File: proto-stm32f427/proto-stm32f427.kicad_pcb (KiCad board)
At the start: 2 copper layers, 54.6 x 66.7 mm, 37 parts, among them J1 Left, J2 Micro_SD_Card, J3 USB, J4 Debug, J5 Right, U1 NCV5501, U2 STM32F427VGTx, Y1 8 MHz

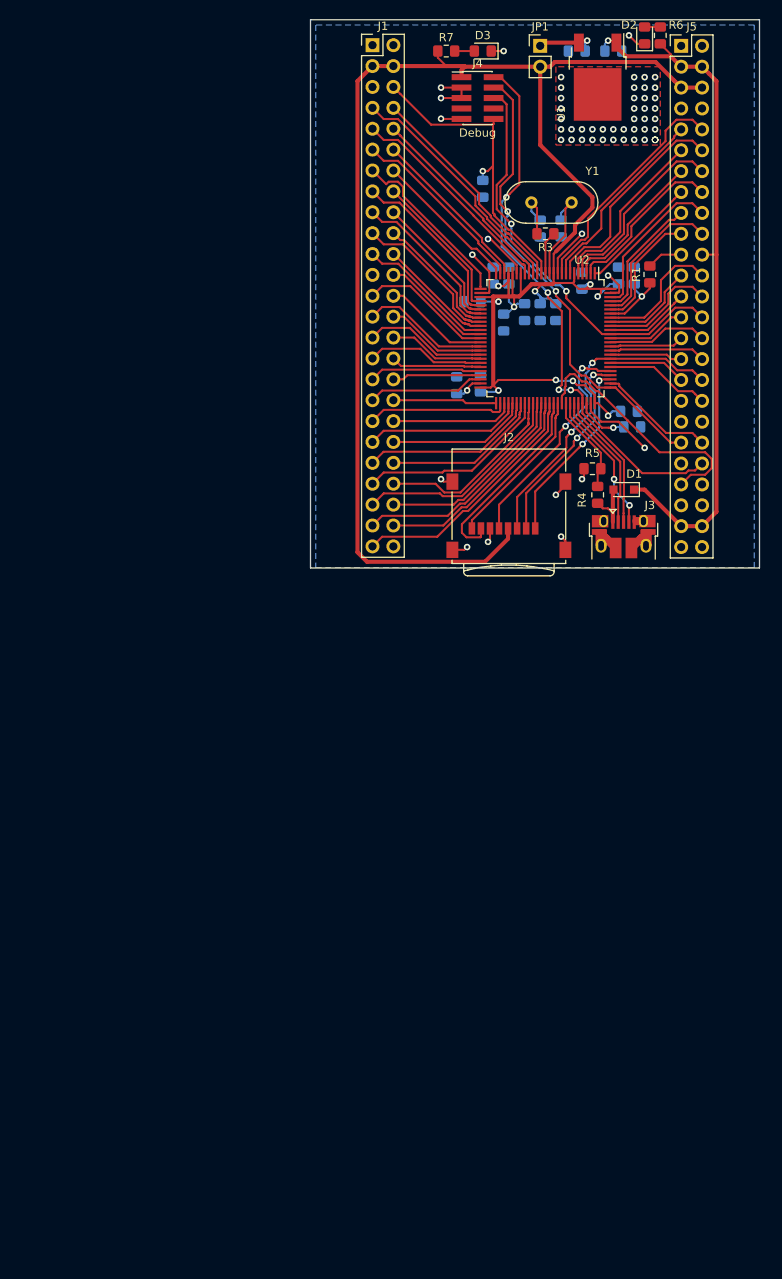
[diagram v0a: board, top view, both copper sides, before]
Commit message: WIP updates for proto board to make smaller
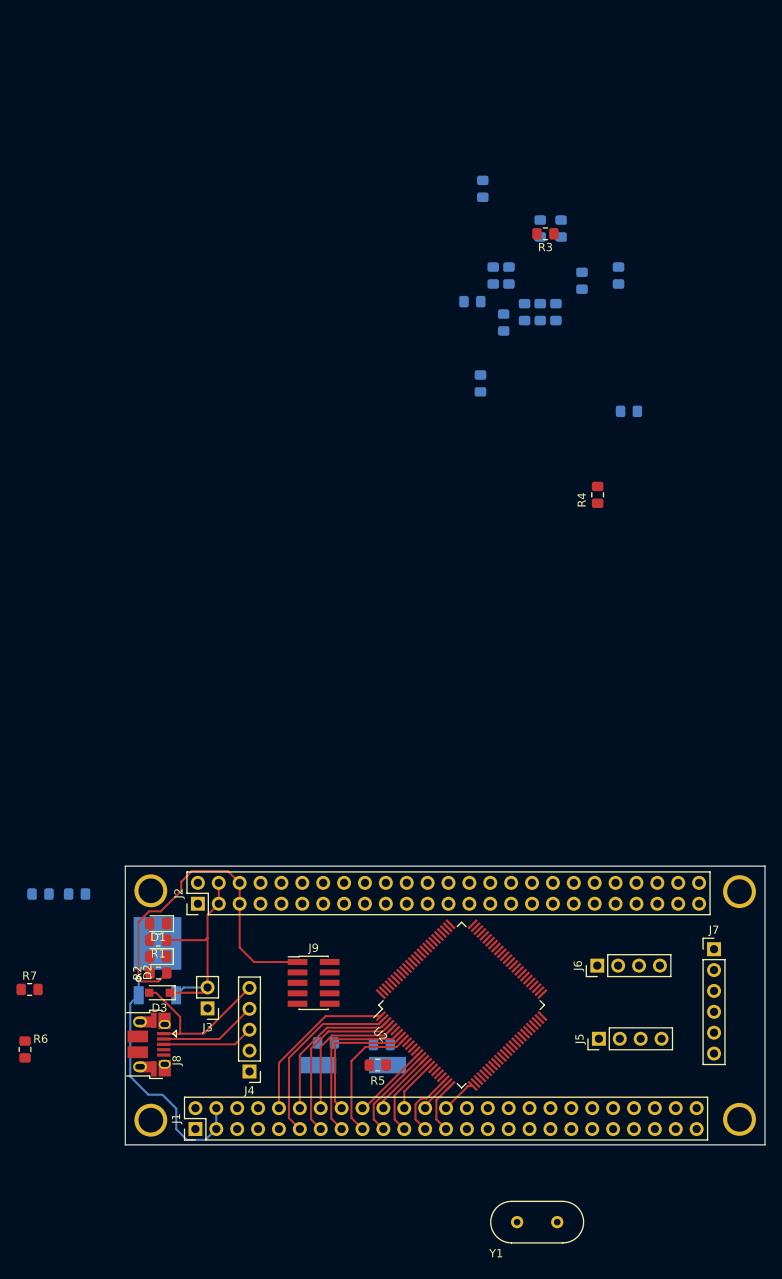
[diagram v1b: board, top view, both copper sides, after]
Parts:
- removed JP1: Idd, Connector_PinHeader_2.54mm:PinHeader_1x02_P2.54mm_Vertical
- added J6: IGNITION, Connector_PinHeader_2.54mm:PinHeader_1x04_P2.54mm_Vertical, F.Cu at (93.3, 136.0)
- added J7: SPI, Connector_PinHeader_2.54mm:PinHeader_1x06_P2.54mm_Vertical, F.Cu at (107.5, 134.0)
- added J8: USB, Connector_USB:USB_Micro-B_Amphenol_10103594-0001LF_Horizontal, F.Cu at (38.8, 145.6)
- added J9: Debug, Connector_PinHeader_1.27mm:PinHeader_2x05_P1.27mm_Vertical_SMD, F.Cu at (58.8, 138.1)
- added REF**: MountingHole_2.5mm_Pad, MountingHole:MountingHole_2.5mm_Pad, F.Cu at (110.6, 127.0)
- added REF**: MountingHole_2.5mm_Pad, MountingHole:MountingHole_2.5mm_Pad, F.Cu at (39.0, 154.8)
- added REF**: MountingHole_2.5mm_Pad, MountingHole:MountingHole_2.5mm_Pad, F.Cu at (110.6, 154.7)
- added REF**: MountingHole_2.5mm_Pad, MountingHole:MountingHole_2.5mm_Pad, F.Cu at (39.0, 126.9)
- added REF**: Crystal_SMD_HC49-SD, Crystal:Crystal_SMD_HC49-SD, B.Cu at (63.5, 148.1)
- C3, C5: value 16 pF -> 2.2 uF
- C4, C6: value 2.2 uF -> 16 pF
- D1: value BAT48JFILM -> LED; footprint Diode_SMD:D_SOD-323_HandSoldering -> LED_SMD:LED_0805_2012Metric_Pad1.15x1.40mm_HandSolder
- D3: value LED -> BAT48JFILM; footprint LED_SMD:LED_0805_2012Metric_Pad1.15x1.40mm_HandSolder -> Diode_SMD:D_SOD-323_HandSoldering
- J2: value Micro_SD_Card -> Right; footprint Connector_Card:microSD_HC_Wuerth_693072010801 -> Connector_PinHeader_2.54mm:PinHeader_2x25_P2.54mm_Vertical
- J3: value USB -> POWER; footprint Connector_USB:USB_Micro-B_Amphenol_10103594-0001LF_Horizontal -> Connector_PinHeader_2.54mm:PinHeader_1x02_P2.54mm_Vertical
- J4: value Debug -> EXTUSB; footprint Connector_PinHeader_1.27mm:PinHeader_2x05_P1.27mm_Vertical_SMD -> Connector_PinHeader_2.54mm:PinHeader_1x05_P2.54mm_Vertical
- J5: value Right -> FUEL; footprint Connector_PinHeader_2.54mm:PinHeader_2x25_P2.54mm_Vertical -> Connector_PinHeader_2.54mm:PinHeader_1x04_P2.54mm_Vertical
- R1: value 1k -> 220
- R2: value 100k -> 220; moved to F.Cu
- R3: value 220 -> 1k
- R4: value 4.7k -> 100k
- R5: value 10k -> 220
- R6: value 220 -> 4.7k
- R7: value 220 -> 10k
- U1: moved to B.Cu
- moved R6 145.5 mm to (23.7, 146.2)
- moved J1 133.6 mm to (44.4, 155.9), turned to 90 degrees
- moved D2 126.7 mm to (39.9, 134.9), turned to 180 degrees
- moved R7 124.9 mm to (24.3, 138.9)
- moved Y1 124.2 mm to (83.5, 167.2), turned to 0 degrees
- moved J4 121.6 mm to (51.0, 148.9), turned to 180 degrees
- moved C1 121.5 mm to (30.0, 127.3)
- moved C2 121.5 mm to (25.6, 127.3)
- moved J5 121.2 mm to (93.5, 144.9), turned to 90 degrees
- moved D3 121.1 mm to (40.0, 139.3)
- moved U1 120.1 mm to (39.8, 135.4), turned to 90 degrees
- moved R2 102.7 mm to (39.9, 136.9), turned to 180 degrees
- moved R1 100.7 mm to (39.9, 132.9), turned to 180 degrees
- moved C6 83.7 mm to (60.3, 145.4)
- moved U2 81.7 mm to (76.8, 140.8), turned to 45 degrees
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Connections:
- C2 pad 1: /3v_regulated -> /3v_cpu
- C3 pad 1: GND -> Net-(C3-Pad1)
- C3 pad 2: /PH0 -> GND
- C4 pad 1: Net-(C4-Pad1) -> GND
- C4 pad 2: GND -> /PH0
- C5 pad 1: GND -> Net-(C5-Pad1)
- C5 pad 2: Net-(C5-Pad2) -> GND
- C6 pad 1: Net-(C6-Pad1) -> GND
- C6 pad 2: GND -> Net-(C6-Pad2)
- D1 pad 1: /5v -> GND
- D1 pad 2: /5v_usb -> Net-(D1-Pad2)
- D3 pad 1: GND -> /5v
- D3 pad 2: Net-(D3-Pad2) -> /5v_usb
- J1 pad 10: /PC2 -> /PE2
- J1 pad 11: /PA1 -> /PE3
- J1 pad 12: /PA0 -> /PE4
- J1 pad 13: /PA3 -> /PE5
- J1 pad 14: /PA2 -> /PE6
- J1 pad 15: /PA5 -> /PC13
- J1 pad 16: /PA4 -> /PC14
- J1 pad 17: /PA7 -> /PC15
- J1 pad 18: /PA6 -> /NRST
- J1 pad 19: /PC5 -> /PC0
- J1 pad 20: /PC4 -> /PC1
- J1 pad 21: /PB1 -> /PC2
- J1 pad 22: /PB0 -> /PC3
- J1 pad 23: GND -> /PA0
- J1 pad 24: /PB2 -> /PA1
- J1 pad 25: /PE7 -> /PA2
- J1 pad 26: /PE8 -> /PA3
- J1 pad 5: GND -> unconnected-(J1-Pad5)
- J1 pad 6: /NRST -> unconnected-(J1-Pad6)
- J1 pad 7: /PC1 -> unconnected-(J1-Pad7)
- J1 pad 8: /PC0 -> unconnected-(J1-Pad8)
- J1 pad 9: /PC3 -> unconnected-(J1-Pad9)
- J2 pad 1: /PC10 -> GND
- J2 pad 2: /PC11 -> GND
- J2 pad 3: /PD2 -> /5v
- J2 pad 4: /3v_cpu -> /5v
- J2 pad 5: /PC12 -> /3v_cpu
- J2 pad 6: GND -> /3v_cpu
- J2 pad 7: /PC8 -> unconnected-(J2-Pad7)
- J2 pad 8: /PC9 -> unconnected-(J2-Pad8)
- J2 pad 9: GND -> /PC14
- J3 pad 1: /5v_usb -> GND
- J3 pad 2: /PA11 -> /5v
- J4 pad 1: /3v_cpu -> GND
- J4 pad 2: /PA13 -> GND
- J4 pad 3: GND -> /PA12
- J4 pad 4: /PA14 -> /PA11
- J4 pad 5: GND -> /5v_usb
- J5 pad 1: GND -> /PD8
- J5 pad 2: GND -> /PD9
- J5 pad 3: /5v -> /PD10
- J5 pad 4: /5v -> /PD11
- R1 pad 1: Net-(R1-Pad1) -> /5v
- R1 pad 2: /BOOT0 -> Net-(D1-Pad2)
- R2 pad 1: GND -> /3v_cpu
- R2 pad 2: Net-(R1-Pad1) -> Net-(D2-Pad2)
- R3 pad 1: /PH1 -> Net-(R3-Pad1)
- R3 pad 2: Net-(C5-Pad2) -> /BOOT0
- R4 pad 1: /PA9 -> GND
- R4 pad 2: /5v_usb -> Net-(R3-Pad1)
- R5 pad 1: /PA9 -> /PH1
- R5 pad 2: GND -> Net-(C6-Pad2)
- R6 pad 1: /5v -> /PA9
- R6 pad 2: Net-(D2-Pad2) -> /5v_usb
- R7 pad 1: /3v_cpu -> /PA9
- R7 pad 2: Net-(D3-Pad2) -> GND
- U1 pad 3: /3v_regulated -> /3v_cpu
- U2 pad 49: Net-(C4-Pad1) -> Net-(C3-Pad1)
- U2 pad 73: Net-(C6-Pad1) -> Net-(C5-Pad1)
- U2 pad 94: Net-(R1-Pad1) -> Net-(R3-Pad1)
- Y1 pad 2: Net-(C5-Pad2) -> Net-(C6-Pad2)
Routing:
- net /3v_cpu: track 246.0 -> 73.2 mm, vias 10 -> 1
- net /PA13: track 67.4 -> 0.00 mm, vias 4 -> 0
- net GND: track 61.9 -> 0.00 mm, vias 58 -> 0
- net /5v: track 85.7 -> 27.5 mm, vias 1 -> 0
- net /PA14: track 57.0 -> 0.00 mm, vias 2 -> 0
- net /PB3: track 50.0 -> 0.00 mm, vias 2 -> 0
- net /PD2: track 39.1 -> 0.00 mm, vias 2 -> 0
- net /PA8: track 31.1 -> 0.00 mm
- net /PC7: track 30.6 -> 0.00 mm
- net /NRST: track 38.0 -> 9.55 mm, vias 1 -> 0
- net /PD15: track 28.4 -> 0.00 mm
- net /PC12: track 28.1 -> 0.00 mm, vias 2 -> 0
- net /PD13: track 26.5 -> 0.00 mm
- net /PC6: track 26.5 -> 0.00 mm
- net /PC11: track 24.6 -> 0.00 mm, vias 2 -> 0
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- removed copper zone on B.Cu, net GND
- removed copper zone on F.Cu, net GND
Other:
- board size 54.6 x 66.7 mm -> 77.8 x 33.9 mm
- net class Default removed
- board text removed: "3v"
- board text removed: "5v"
- board text removed: "A0"
- board text removed: "A1"
- board text removed: "A13"
- board text removed: "A14"
- board text removed: "A15"
- board text removed: "A2"
- board text removed: "A3"
- board text removed: "A4"
- board text removed: "A5"
- board text removed: "A6"
- board text removed: "A7"
- board text removed: "A8"
- board text removed: "B0"
- board text removed: "B1"
- board text removed: "B10"
- board text removed: "B11"
- board text removed: "B12"
- board text removed: "B13"
- board text removed: "B14"
- board text removed: "B15"
- board text removed: "B2"
- board text removed: "B3"
- board text removed: "B4"
- board text removed: "B5"
- board text removed: "B6"
- board text removed: "B7"
- board text removed: "B8"
- board text removed: "B9"
- board text removed: "BOOT0"
- board text removed: "C0"
- board text removed: "C1"
- board text removed: "C13"
- board text removed: "C14"
- board text removed: "C15"
- board text removed: "C2"
- board text removed: "C3"
- board text removed: "C4"
- board text removed: "C5"
- board text removed: "C6"
- board text removed: "C7"
- board text removed: "D0"
- board text removed: "D1"
- board text removed: "D10"
- board text removed: "D11"
- board text removed: "D12"
- board text removed: "D13"
- board text removed: "D14"
- board text removed: "D15"
- board text removed: "D2"
- board text removed: "D3"
- board text removed: "D4"
- board text removed: "D5"
- board text removed: "D6"
- board text removed: "D7"
- board text removed: "D8"
- board text removed: "D9"
- board text removed: "E0"
- board text removed: "E1"
- board text removed: "E10"
- board text removed: "E11"
- board text removed: "E12"
- board text removed: "E13"
- board text removed: "E14"
- board text removed: "E15"
- board text removed: "E2"
- board text removed: "E3"
- board text removed: "E4"
- board text removed: "E5"
- board text removed: "E6"
- board text removed: "E7"
- board text removed: "E8"
- board text removed: "E9"
- board text removed: "GND"
- board text removed: "RST"
